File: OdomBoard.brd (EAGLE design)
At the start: 160 x 100 mm, 36 parts, among them CN1 8P8C-LED, J1 EP2.5-4-SIDE, J2 EP2.5-4-SIDE, J3 EP2.5-4-SIDE, SW1 SWITCH_TACTILETOP, U1 STM32F103C8, U2 NCV7351D1E, U6 MC34063AD, U7 XC6206

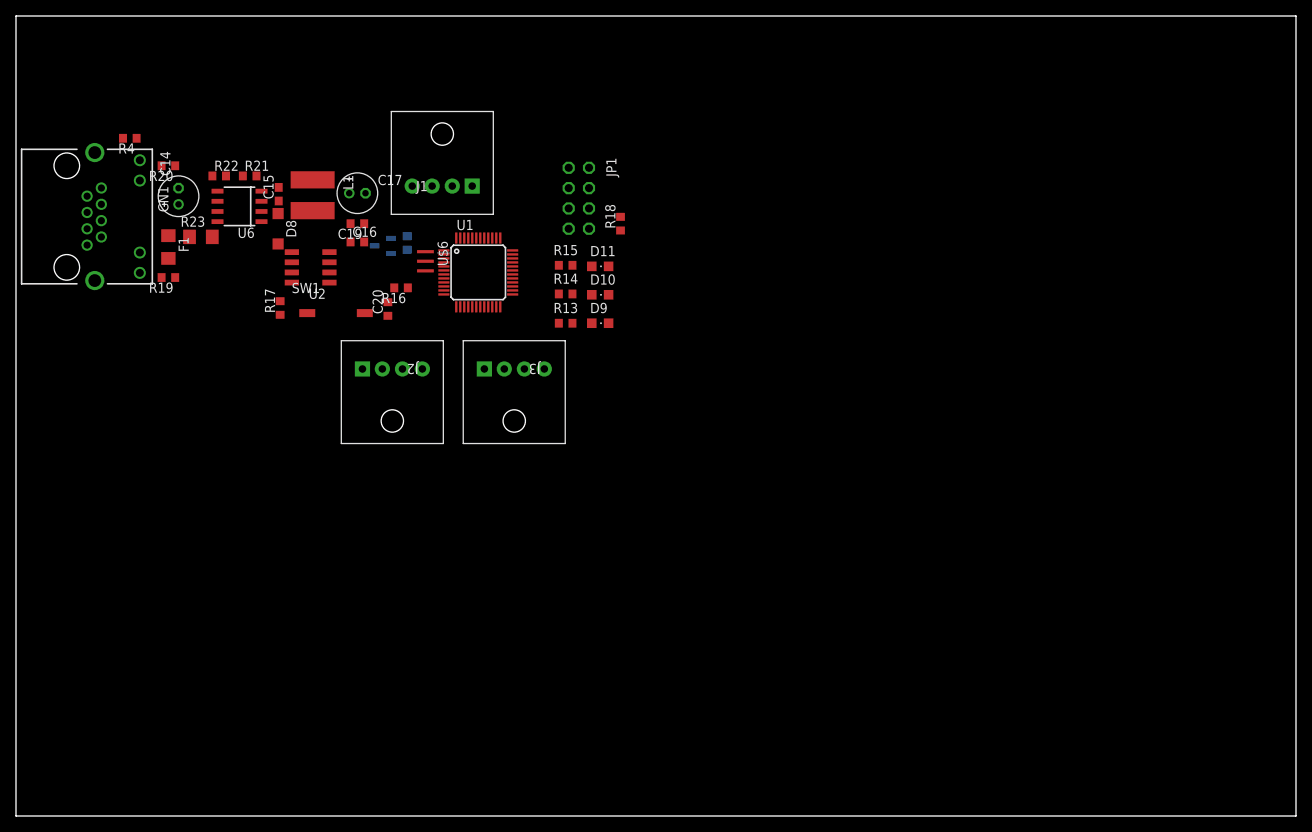
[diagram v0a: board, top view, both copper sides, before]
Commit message: First Version
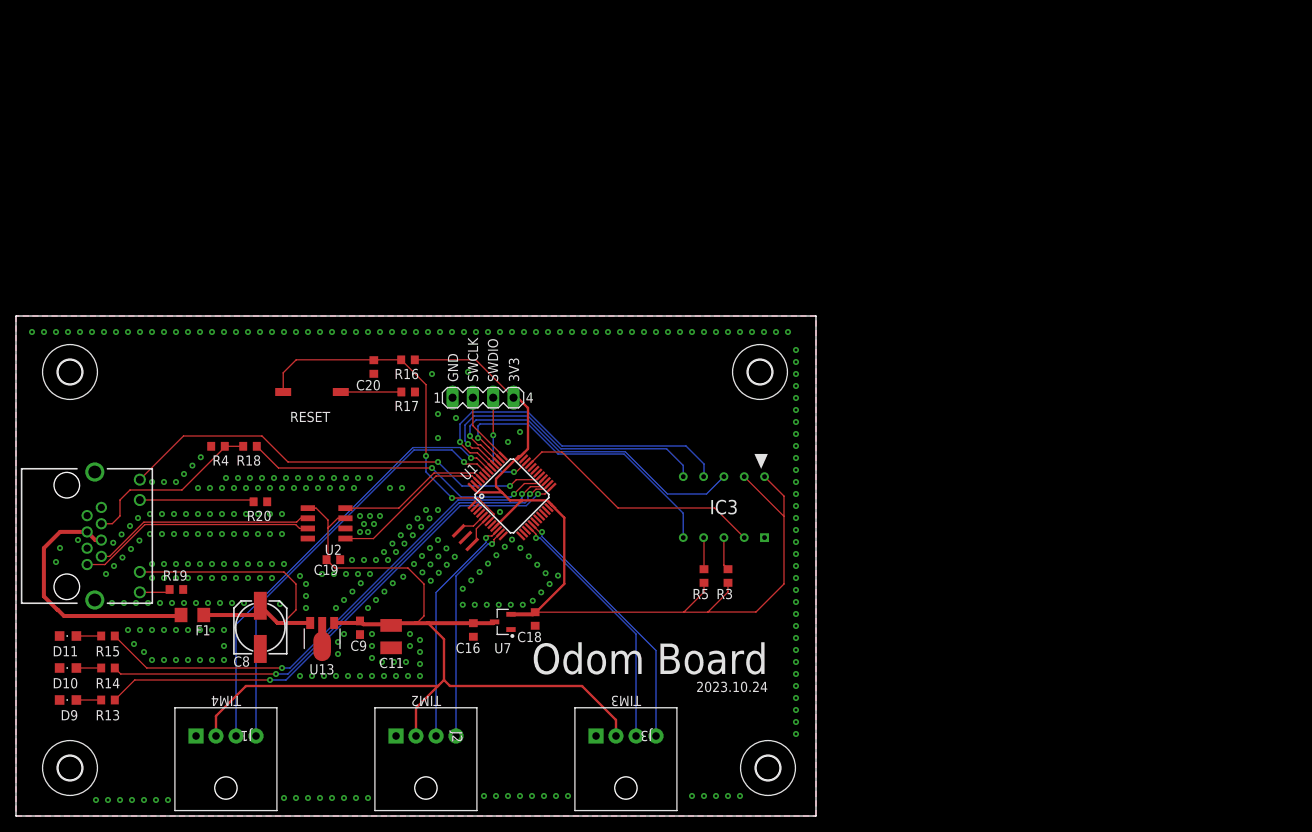
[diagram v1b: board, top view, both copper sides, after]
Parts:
- removed C14, C17: 22u, rcl:E2-5
- removed C15: 220p, rcl:C0603
- removed D8: (no value), diode:SOD123
- removed JP1: (no value), pinhead:2X04
- removed L1: 220u, l_ysk:L5852
- removed R21: 3.6k, rcl:R0603
- removed R22: 1.2k, rcl:R0603
- removed R23: 0.68, rcl:R1206
- removed U6: MC34063AD, mc34063:SOIC8
- added C11: 10u, rcl:C1210
- added C8: EEEHA1E220P, rcl:153CLV-0605
- added C9: 100n, rcl:C0603
- added H1, H2, H3, H4: MOUNT-HOLE3.0, CRS_EAGLE_Lib:3,0
- added IC3: MPU-9250_MOD, CRS_EAGLE_Lib:MPU_9250_MOD
- added R3, R5: 4.7k, rcl:R0603
- added SV1: (no value), con-lstb:MA04-1
- added U13: 78L05F, linear:SOT89
- moved D9 81.5 mm to (6.50, 14.5), turned to 90 degrees
- moved D10 81.3 mm to (6.50, 18.5), turned to 90 degrees
- moved D11 81.0 mm to (6.50, 22.5), turned to 90 degrees
- moved R13 74.1 mm to (11.5, 14.5), turned to 180 degrees
- moved R14 73.9 mm to (11.5, 18.5), turned to 180 degrees
- moved R15 73.6 mm to (11.5, 22.5), turned to 180 degrees
- moved J1 71.5 mm to (30.0, 10.0), turned to 180 degrees
- moved R18 54.0 mm to (29.2, 46.2), turned to 180 degrees
- moved C16 50.6 mm to (57.2, 23.3), turned to 270 degrees
- moved C18 49.6 mm to (64.9, 24.6), flipped to the top, turned to 270 degrees
- moved U7 49.3 mm to (60.8, 24.3), flipped to the top, turned to 180 degrees
- moved J3 48.0 mm to (80.0, 10.0)
- moved F1 46.1 mm to (22.1, 25.1), turned to 180 degrees
- moved J2 46.1 mm to (55.0, 10.0)
- moved R20 43.5 mm to (30.6, 39.3)
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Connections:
- net CANH renamed CAN_PAIR_P
- net CANL renamed CAN_PAIR_N
- removed net +24V: C14.+, CN1.GA, F1.1, R23.1, U6.6
- removed net N$13: R23.2, U6.1, U6.7, U6.8
- removed net N$14: D8.C, L1.P$1, U6.2
- removed net N$15: C15.1, U6.3
- removed net N$17: R21.1, R22.2, U6.5
- removed net UART_RX: JP1.1
- removed net UART_TX: JP1.3
- new net +12V: C8.+, CN1.GA, F1.1, U13.3
- new net MPU_INT: IC3.9, U1.33
- new net N$3: IC3.8, R3.1
- new net N$4: IC3.7, R5.1
- net +3V3: now also IC3.1, IC3.2, R3.2, R5.2, SV1.4; no longer JP1.8
- net +5V: now also C11.2, C9.1, U13.1; no longer C17.+, JP1.5, L1.P$2, R21.2
- net GNDIO: now also C11.1, C8.-, C9.2, IC3.10, SV1.1, U13.2, U13.2@1; no longer C14.-, C15.2, C17.-, D8.A, JP1.2, JP1.7, R22.1, U6.4
- net SPI1_CS: now also IC3.6
- net SPI1_MISO: now also IC3.5
- net SPI1_MOSI: now also IC3.4
- net SPI1_SCK: now also IC3.3
- net SWCLK: now also SV1.2; no longer JP1.4
- net SWDIO: now also SV1.3; no longer JP1.6
- net TIM3_CH1: now also J3.3, U1.16; no longer J3.4, U1.17
- net TIM3_CH2: now also J3.4, U1.17; no longer J3.3, U1.16
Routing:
- net +3V3: track 0.00 -> 127.0 mm
- net +5V: track 0.00 -> 124.1 mm
- net LED0: track 0.00 -> 65.7 mm, vias 0 -> 2
- net LED2: track 0.00 -> 65.5 mm, vias 0 -> 2
- net LED1: track 0.00 -> 64.7 mm, vias 0 -> 2
- net TIM4_CH1: track 0.00 -> 55.9 mm, vias 0 -> 1
- net LED_CAN: track 0.00 -> 55.5 mm, vias 0 -> 2
- net TIM4_CH2: track 0.00 -> 54.2 mm, vias 0 -> 1
- net !RESET: track 0.00 -> 45.1 mm, vias 0 -> 2
- net SPI1_MOSI: track 0.00 -> 43.0 mm, vias 0 -> 1
- net SPI1_SCK: track 0.00 -> 42.9 mm, vias 0 -> 1
- net +12V: track 0.00 -> 40.6 mm
- net !EMS: track 0.00 -> 39.4 mm, vias 0 -> 2
- net SPI1_CS: track 0.00 -> 38.8 mm, vias 0 -> 1
- net SPI1_MISO: track 0.00 -> 38.6 mm, vias 0 -> 1
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- added copper zone on layer 1, net GNDIO
- added copper zone on layer 16, net GNDIO
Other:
- board size 160 x 100 mm -> 100 x 62.5 mm
- board text added: "2023.10.24"
- board text added: "3V3"
- board text added: "GND"
- board text added: "Odom Board"
- board text added: "RESET"
- board text added: "SWCLK"
- board text added: "SWDIO"
- board text added: "TIM2"
- board text added: "TIM3"
- board text added: "TIM4"
